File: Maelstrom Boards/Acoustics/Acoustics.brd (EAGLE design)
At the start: 100 x 80 mm, 175 parts

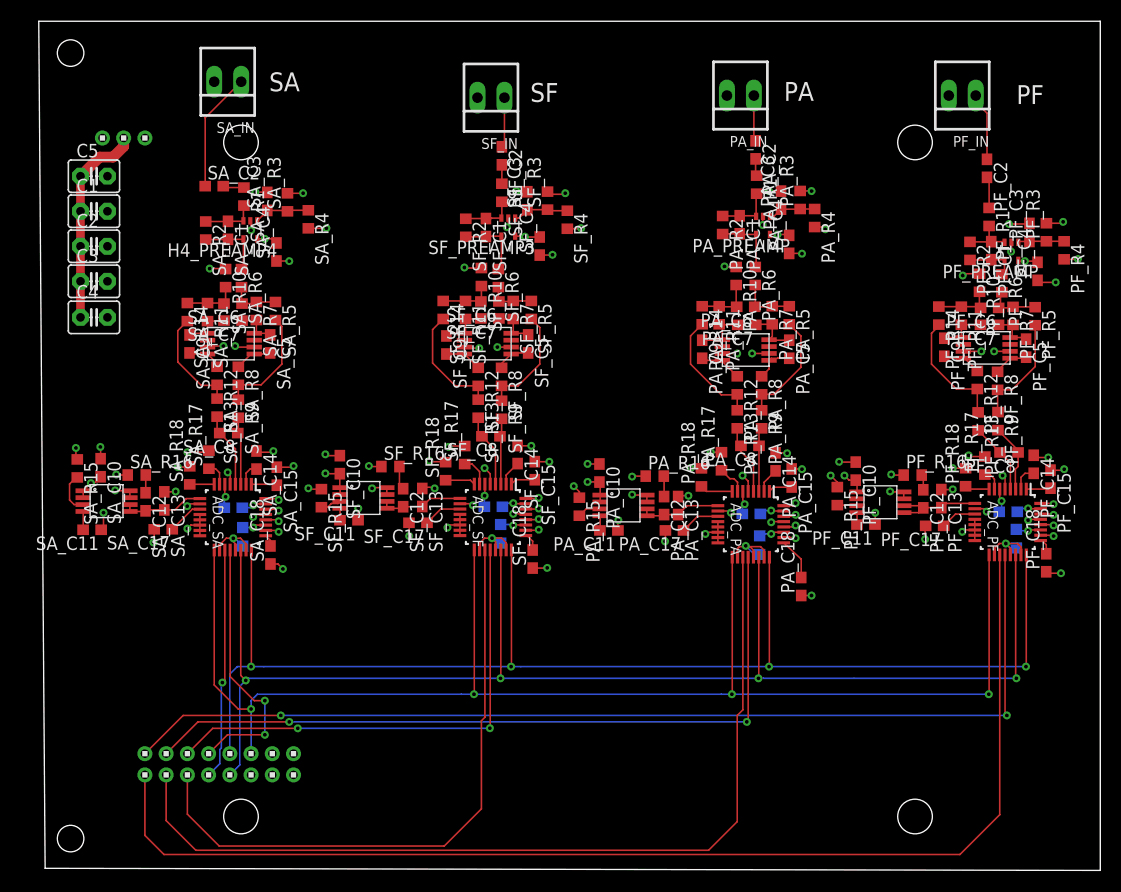
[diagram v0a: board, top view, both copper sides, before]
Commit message: Prettying things up
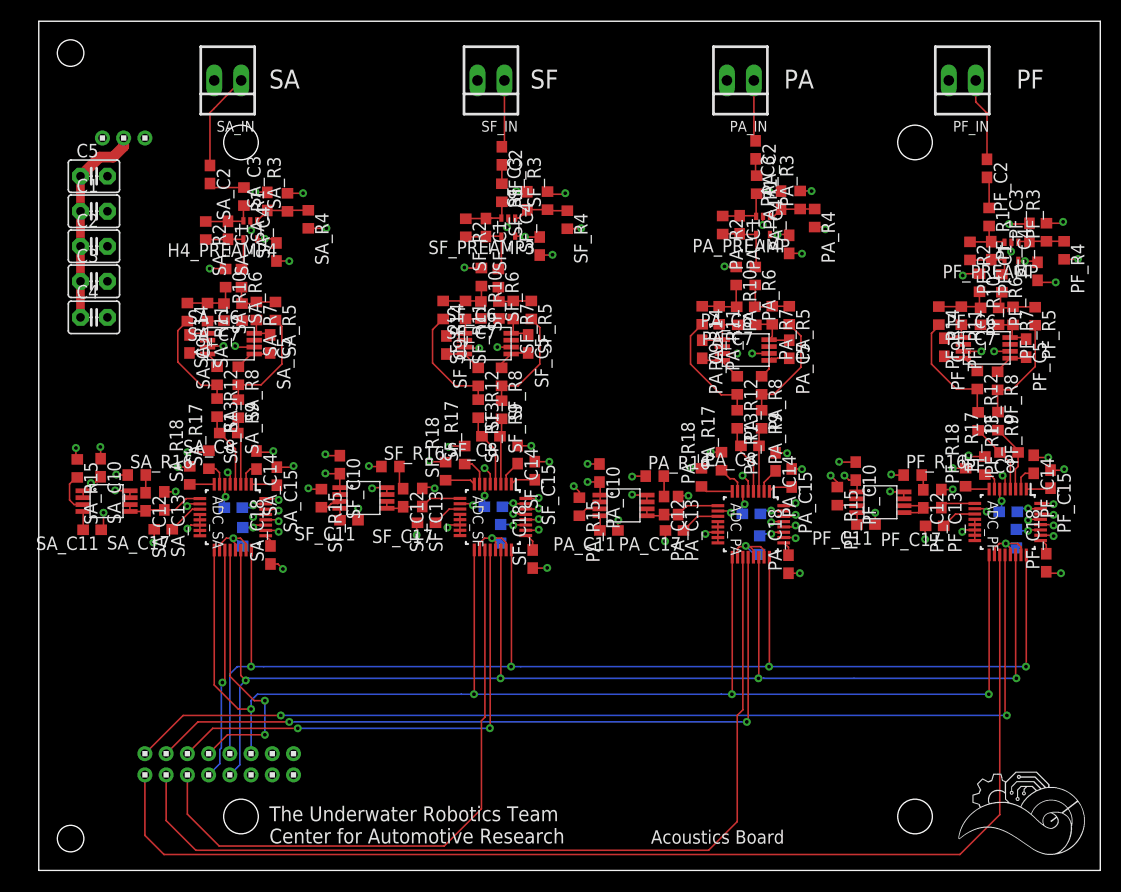
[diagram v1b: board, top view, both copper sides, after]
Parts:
- moved PA_C18 2.42 mm to (70.6, 28.8)
- moved SF_IN 1.62 mm to (42.6, 74.4)
- moved PA_IN 1.42 mm to (66.1, 74.4)
- moved PF_IN 1.42 mm to (87.0, 74.4)
- moved SA_C2 1.17 mm to (16.1, 65.6), turned to 270 degrees
- moved SF_C17 0.80 mm to (36.5, 32.8)
- moved SA_IN 0.12 mm to (17.8, 74.4)
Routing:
- net N$149: track 3.98 -> 1.36 mm
- net RAW_SA: track 11.2 -> 9.20 mm
- net RAW_SF: track 4.73 -> 6.35 mm
- net RAW_PF: track 6.45 -> 7.87 mm
- net RAW_PA: track 4.33 -> 5.76 mm
- net N$145: track 1.97 -> 3.36 mm
- net N$159: track 3.64 -> 2.84 mm
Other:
- outline, holes or cut-outs redrawn
- board text added: "Acoustics Board"
- board text added: "The Underwater Robotics Team Center for Automotive Research"
